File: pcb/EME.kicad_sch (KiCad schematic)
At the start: 50 parts, among them J1 BMP180, J10 Reset, J11 UART0, J12 SPI_CONN, J13 UART2, J14 MQ135, J2 ReedSwitchX8, J3 SS41, J4 Hoja Mojada, J5 PanelSolar, J6 BH1750, J7 DHT22, J8 Baterias, J9 Jumper, SW1 Enable, U1 LM78M05_TO220, U5 TL082

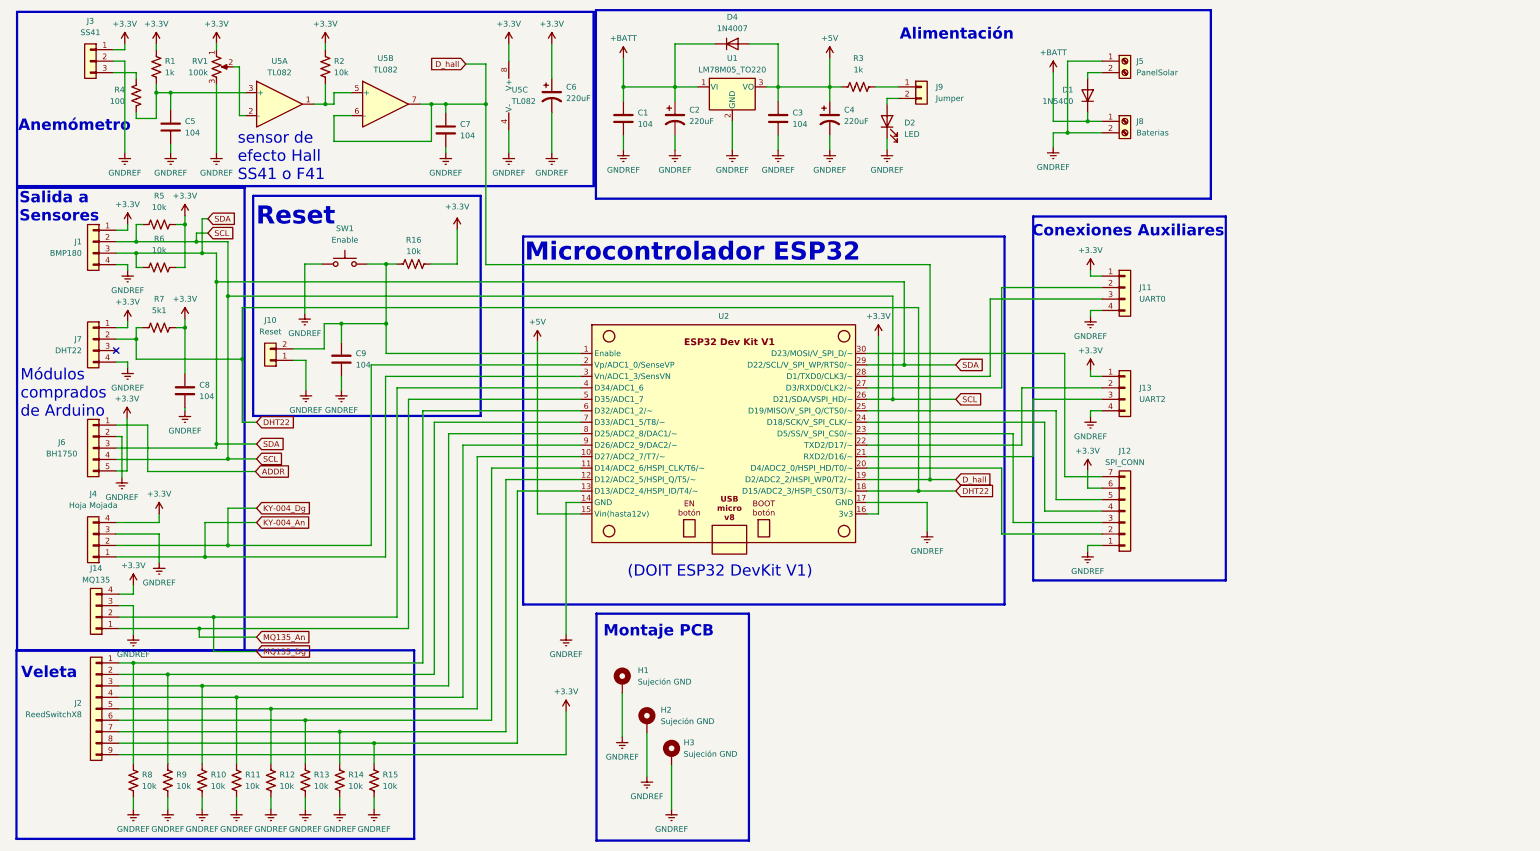
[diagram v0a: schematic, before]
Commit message: Add files via upload
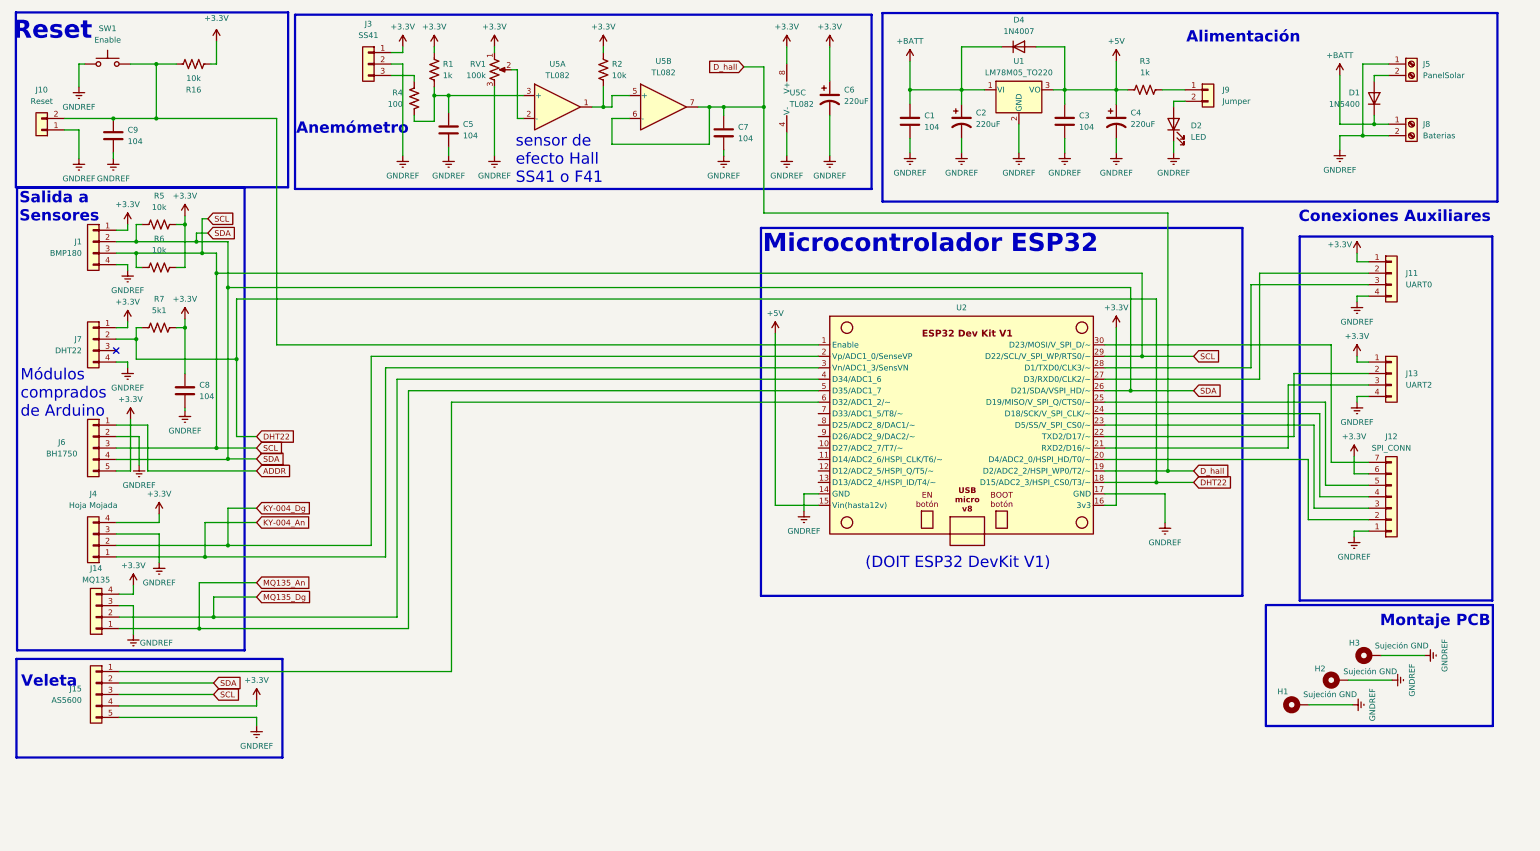
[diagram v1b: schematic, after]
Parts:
- removed J2: ReedSwitchX8, Connector_PinHeader_2.54mm:PinHeader_1x09_P2.54mm_Vertical, symbol Connector_Generic:Conn_01x09
- removed R10, R11, R12, R13, R14, R15, R8, R9: 10k, Resistor_THT:R_Axial_DIN0207_L6.3mm_D2.5mm_P10.16mm_Horizontal, symbol Device:R_US
- added J15: AS5600, Connector_PinHeader_2.54mm:PinHeader_1x05_P2.54mm_Vertical, symbol Connector_Generic:Conn_01x05
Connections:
- net +3.3V: now also J15.4 (Pin_4)
- net GNDREF: now also J15.5 (Pin_5)
- net SCL: now also J1.3 (Pin_3), J6.3 (Pin_3), R6.1, U2.29 (D22/SCL/V_SPI_WP/RTS0/~), J15.3 (Pin_3); no longer J1.2 (Pin_2), J6.4 (Pin_4), R5.1, U2.26 (D21/SDA/VSPI_HD/~)
- net SDA: now also J1.2 (Pin_2), J6.4 (Pin_4), R5.1, U2.26 (D21/SDA/VSPI_HD/~), J15.2 (Pin_2); no longer J1.3 (Pin_3), J6.3 (Pin_3), R6.1, U2.29 (D22/SCL/V_SPI_WP/RTS0/~)
- net at U2.6 (D32/ADC1_2/~): now also J15.1 (Pin_1)
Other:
- moved on the sheet: C1, C2, C3, C4, C5, C6, C7, C9, D1, D2, D4, H1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

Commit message: se actualizó la PCB
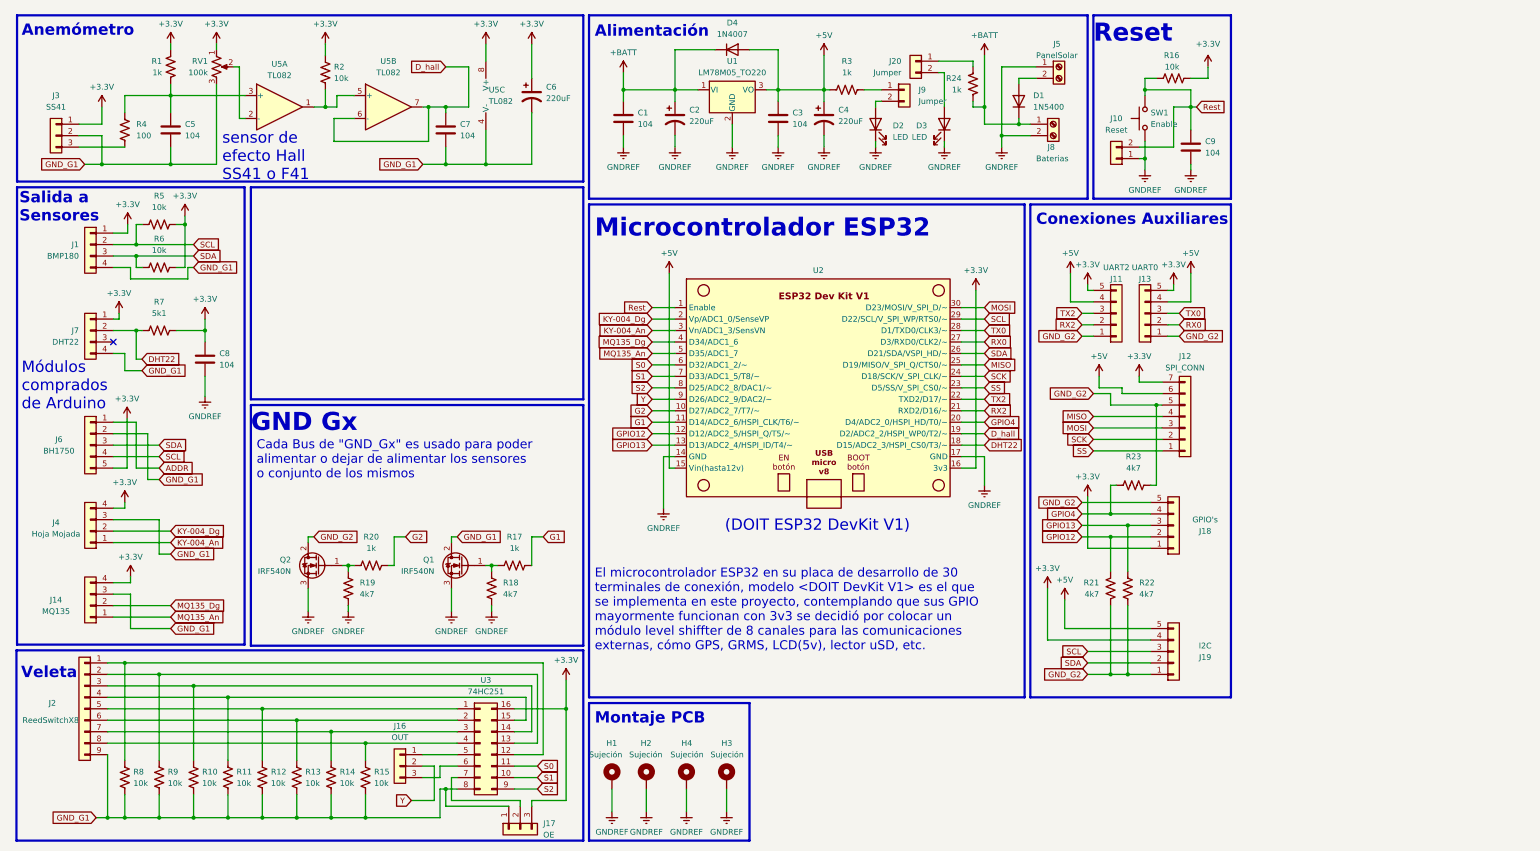
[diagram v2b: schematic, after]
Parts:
- removed J11: UART0, Connector_PinHeader_2.54mm:PinHeader_1x04_P2.54mm_Vertical, symbol Connector_Generic:Conn_01x04
- removed J13: UART2, Connector_PinHeader_2.54mm:PinHeader_1x04_P2.54mm_Vertical, symbol Connector_Generic:Conn_01x04
- removed J15: AS5600, Connector_PinHeader_2.54mm:PinHeader_1x05_P2.54mm_Vertical, symbol Connector_Generic:Conn_01x05
- added D3: LED, LED_THT:LED_D5.0mm_Clear, symbol Device:LED
- added H4: Sujeción, MountingHole:MountingHole_3.2mm_M3_Pad_Via, symbol Mechanical:MountingHole_Pad_MP
- added J11: UART2, Connector_PinHeader_2.54mm:PinHeader_1x05_P2.54mm_Vertical, symbol Connector_Generic:Conn_01x05
- added J13: UART0, Connector_PinHeader_2.54mm:PinHeader_1x05_P2.54mm_Vertical, symbol Connector_Generic:Conn_01x05
- added J16: OUT, Connector_PinHeader_2.54mm:PinHeader_1x03_P2.54mm_Vertical, symbol Connector_Generic:Conn_01x03
- added J17: OE, Connector_PinHeader_2.54mm:PinHeader_1x03_P2.54mm_Vertical, symbol Connector_Generic:Conn_01x03
- added J18: GPIO's, Connector_PinHeader_2.54mm:PinHeader_1x05_P2.54mm_Vertical, symbol Connector_Generic:Conn_01x05
- added J19: I2C, Connector_PinHeader_2.54mm:PinHeader_1x05_P2.54mm_Vertical, symbol Connector_Generic:Conn_01x05
- added J2: ReedSwitchX8, Connector_PinHeader_2.54mm:PinHeader_1x09_P2.54mm_Vertical, symbol Connector_Generic:Conn_01x09
- added J20: Jumper, Connector_PinHeader_2.54mm:PinHeader_1x02_P2.54mm_Vertical, symbol Connector_Generic:Conn_01x02
- added Q1, Q2: IRF540N, Package_TO_SOT_THT:TO-220-3_Vertical, symbol Transistor_FET:IRF540N
- added R10, R11, R12, R13, R14, R15, R8, R9: 10k, Resistor_THT:R_Axial_DIN0207_L6.3mm_D2.5mm_P10.16mm_Horizontal, symbol Device:R_US
- added R17, R20, R24: 1k, Resistor_THT:R_Axial_DIN0207_L6.3mm_D2.5mm_P10.16mm_Horizontal, symbol Device:R_US
- added R18, R19, R21, R22, R23: 4k7, Resistor_THT:R_Axial_DIN0207_L6.3mm_D2.5mm_P10.16mm_Horizontal, symbol Device:R_US
- added U3: 74HC251, Package_DIP:DIP-16_W7.62mm_LongPads, symbol Connector_Generic:Conn_02x08_Counter_Clockwise
- H1, H2, H3: value Sujeción GND -> Sujeción
- J5: footprint TerminalBlock_Phoenix:TerminalBlock_Phoenix_MPT-0,5-2-2.54_1x02_P2.54mm_Horizontal -> TerminalBlock_Phoenix:TerminalBlock_Phoenix_PT-1,5-2-3.5-H_1x02_P3.50mm_Horizontal
- J8: footprint TerminalBlock_Phoenix:TerminalBlock_Phoenix_MPT-0,5-2-2.54_1x02_P2.54mm_Horizontal -> TerminalBlock_Phoenix:TerminalBlock_Phoenix_PT-1,5-2-5.0-H_1x02_P5.00mm_Horizontal
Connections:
- net +3.3V: now also J12.7 (Pin_7), R16.2, J11.5 (Pin_5), J13.5 (Pin_5), J17.3 (Pin_3), J18.1 (Pin_1), J19.4 (Pin_4), U3.16 (Pin_16); no longer J12.6 (Pin_6), R16.1
- net +5V: now also J12.6 (Pin_6), J11.4 (Pin_4), J13.4 (Pin_4), J19.5 (Pin_5)
- net +BATT: now also R24.1
- net GNDREF: now also D3.1 (K), H4.MP, Q1.3 (S), Q2.3 (S), R18.1, R19.1; no longer C5.2, C6.2, C7.2, J1.4 (Pin_4), J12.1 (Pin_1), J14.3 (Pin_3), J3.2 (Pin_2), J4.3 (Pin_3), J6.2 (Pin_2), J7.4 (Pin_4), RV1.3, U5.4 (V-)
- net SCL: now also J1.2 (Pin_2), J6.4 (Pin_4), R5.1, J19.3 (Pin_3); no longer J1.3 (Pin_3), J6.3 (Pin_3), R6.1
- net SDA: now also J1.3 (Pin_3), J6.3 (Pin_3), R6.1, J19.2 (Pin_2); no longer J1.2 (Pin_2), J6.4 (Pin_4), R5.1
- net GPIO4: now reaches U2.20 (D4/ADC2_0/HSPI_HD/T0/~)
- net GPIO4: now also J18.4 (Pin_4), R23.2; no longer J12.2 (Pin_2)
- net MOSI: now reaches J12.3 (Pin_3)
- net MOSI: now also U2.30 (D23/MOSI/V_SPI_D/~); no longer U2.23 (D5/SS/V_SPI_CS0/~)
- net MISO: now reaches J12.4 (Pin_4)
- net MISO: now also U2.25 (D19/MISO/V_SPI_Q/CTS0/~); no longer U2.24 (D18/SCK/V_SPI_CLK/~)
- net GND_G2: now reaches J12.5 (Pin_5)
- net GND_G2: now also J11.1 (Pin_1), J13.1 (Pin_1), J18.5 (Pin_5), J19.1 (Pin_1), Q2.2 (D), R21.1, R22.1, R23.1; no longer U2.25 (D19/MISO/V_SPI_Q/CTS0/~)
- net at C5.1, R1.2, U5.3 (+): now also R4.1; no longer R4.2
- net Rest: now reaches C9.1, J10.2 (Pin_2), SW1.2, U2.1 (Enable)
- net Rest: now also R16.1; no longer R16.2
- net RX0: now reaches U2.27 (D3/RXD0/CLK2/~)
- net RX0: now also J13.2 (Pin_2)
- net TX0: now reaches U2.28 (D1/TXD0/CLK3/~)
- net TX0: now also J13.3 (Pin_3)
- net at J3.3 (Pin_3): now also R4.2; no longer R4.1
- net G2: now reaches U2.10 (D27/ADC2_7/T7/~)
- net G2: now also R20.2
- net G1: now reaches U2.11 (D14/ADC2_6/HSPI_CLK/T6/~)
- net G1: now also R17.2
- net GPIO12: now reaches U2.12 (D12/ADC2_5/HSPI_Q/T5/~)
- net GPIO12: now also J18.2 (Pin_2), R21.2
- net GPIO13: now reaches U2.13 (D13/ADC2_4/HSPI_ID/T4/~)
- net GPIO13: now also J18.3 (Pin_3), R22.2
- net RX2: now reaches U2.21 (RXD2/D16/~)
- net RX2: now also J11.2 (Pin_2)
- net TX2: now reaches U2.22 (TXD2/D17/~)
- net TX2: now also J11.3 (Pin_3)
- net S0: now reaches U2.6 (D32/ADC1_2/~)
- net S0: now also U3.11 (Pin_11)
- net S1: now reaches U2.7 (D33/ADC1_5/T8/~)
- net S1: now also U3.10 (Pin_10)
- net S2: now reaches U2.8 (D25/ADC2_8/DAC1/~)
- net S2: now also U3.9 (Pin_9)
- net Y: now reaches U2.9 (D26/ADC2_9/DAC2/~)
- net Y: now also J16.2 (Pin_2)
- new net: J2.3 (Pin_3), R10.1, U3.14 (Pin_14)
- new net: Q1.1 (G), R17.1, R18.2
- new net: J2.4 (Pin_4), R11.1, U3.15 (Pin_15)
- new net: J2.8 (Pin_8), R15.1, U3.4 (Pin_4)
- new net: J2.2 (Pin_2), R9.1, U3.13 (Pin_13)
- new net: J2.6 (Pin_6), R13.1, U3.2 (Pin_2)
- new net: J2.1 (Pin_1), R8.1, U3.12 (Pin_12)
- new net: Q2.1 (G), R19.2, R20.1
- new net: J2.7 (Pin_7), R14.1, U3.3 (Pin_3)
- new net: J20.1 (Pin_1), R24.2
- new net: D3.2 (A), J20.2 (Pin_2)
- new net: J2.5 (Pin_5), R12.1, U3.1 (Pin_1)
- new net: J16.1 (Pin_1), U3.5 (Pin_5)
- new net: J16.3 (Pin_3), U3.6 (Pin_6)
- new net: J17.2 (Pin_2), U3.7 (Pin_7)
- new net GND_G1: C5.2, C6.2, C7.2, J1.4 (Pin_4), J14.3 (Pin_3), J17.1 (Pin_1), J2.9 (Pin_9), J3.2 (Pin_2), J4.3 (Pin_3), J6.2 (Pin_2), J7.4 (Pin_4), Q1.2 (D), R10.2, R11.2, R12.2, R13.2, R14.2, R15.2, R8.2, R9.2, RV1.3, U3.8 (Pin_8), U5.4 (V-)
- new net SCK: J12.2 (Pin_2), U2.24 (D18/SCK/V_SPI_CLK/~)
- new net SS: J12.1 (Pin_1), U2.23 (D5/SS/V_SPI_CS0/~)
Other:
- note added: "Cada Bus de "GND_Gx" es usado para poder alimentar o dejar de alimentar los sensores o conjunto de los mismos"
- note added: "El microcontrolador ESP32 en su placa de desarrollo de 30 terminales de conexión, modelo <DOIT DevKit V1> es el que se implementa en este proyecto, contemplando que sus GPIO mayormente funcionan con 3v3 se decidió por colocar un módulo level shiffter de 8 canales para las comunicaciones externas, cómo GPS, GRMS, LCD(5v), lector uSD, etc."
- note added: "GND Gx"
- moved on the sheet: C1, C2, C3, C4, C5, C6, C7, C8, C9, D1, D2, D4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

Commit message: se actualizó la PCB
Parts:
- J5: footprint TerminalBlock_Phoenix:TerminalBlock_Phoenix_PT-1,5-2-3.5-H_1x02_P3.50mm_Horizontal -> TerminalBlock_Phoenix:TerminalBlock_Phoenix_PT-1,5-2-5.0-H_1x02_P5.00mm_Horizontal
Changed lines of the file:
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@@
 			)
 		)
-		(property "Footprint" "TerminalBlock_Phoenix:TerminalBlock_Phoenix_PT-1,5-2-3.5-H_1x02_P3.50mm_Horizontal"
+		(property "Footprint" "TerminalBlock_Phoenix:TerminalBlock_Phoenix_PT-1,5-2-5.0-H_1x02_P5.00mm_Horizontal"
 			(at 245.11 25.4 0)
 			(effects
